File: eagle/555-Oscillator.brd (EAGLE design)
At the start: 27.9 x 30.5 mm, 8 parts, among them IC1 555

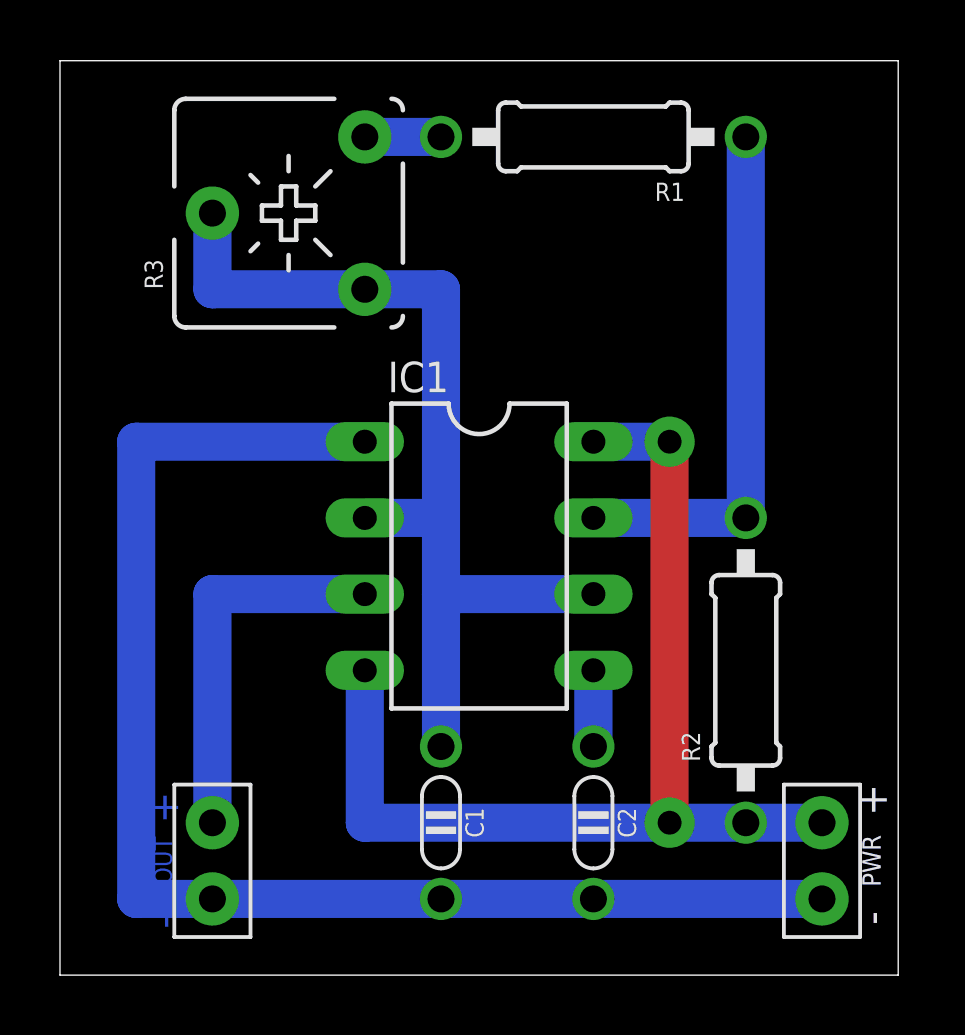
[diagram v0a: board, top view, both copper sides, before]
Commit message: ...
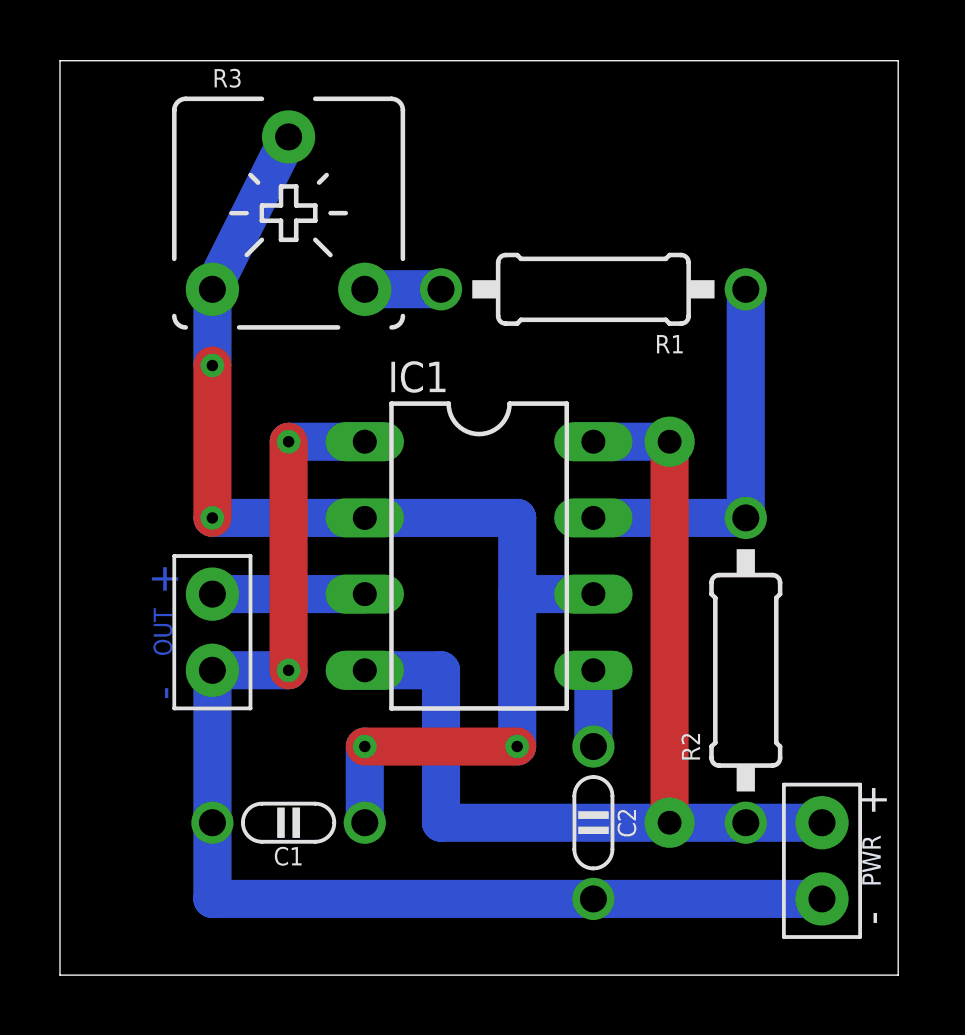
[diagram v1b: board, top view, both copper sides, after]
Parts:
- moved OUT 7.62 mm to (5.08, 11.4)
- moved R1 5.08 mm to (17.8, 22.9)
- moved C1 5.08 mm to (7.62, 5.08), turned to 90 degrees
- turned R3 to 0 degrees
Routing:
- net N$3: track 33.0 -> 41.2 mm, vias 0 -> 4
- net N$8: track 12.7 -> 5.08 mm
- net GND: track 45.7 -> 40.6 mm, vias 0 -> 2
- net N$1: track 17.8 -> 12.7 mm
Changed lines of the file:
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@@
 <layer number="24" name="bOrigins" color="15" fill="1" visible="yes" active="yes"/>
 <layer number="25" name="tNames" color="7" fill="1" visible="yes" active="yes"/>
-<layer number="26" name="bNames" color="7" fill="1" visible="no" active="yes"/>
+<layer number="26" name="bNames" color="7" fill="1" visible="yes" active="yes"/>
 <layer number="27" name="tValues" color="7" fill="1" visible="yes" active="yes"/>
-<layer number="28" name="bValues" color="7" fill="1" visible="no" active="yes"/>
+<layer number="28" name="bValues" color="7" fill="1" visible="yes" active="yes"/>
 <layer number="29" name="tStop" color="7" fill="3" visible="no" active="yes"/>
 <layer number="30" name="bStop" color="7" fill="6" visible="no" active="yes"/>
@@
 <layer number="46" name="Milling" color="3" fill="1" visible="no" active="yes"/>
 <layer number="47" name="Measures" color="7" fill="1" visible="no" active="yes"/>
-<layer number="48" name="Document" color="7" fill="1" visible="yes" active="yes"/>
+<layer number="48" name="Document" color="7" fill="1" visible="no" active="yes"/>
 <layer number="49" name="Reference" color="7" fill="1" visible="no" active="yes"/>
 <layer number="50" name="dxf" color="7" fill="1" visible="no" active="yes"/>
@@
 </autorouter>
 <elements>
-<element name="C1" library="c" package="C050-020X036/V" value="470n" x="12.7" y="5.08" rot="R180"/>
+<element name="C1" library="c" package="C050-020X036/V" value="470n" x="7.62" y="5.08" rot="R90"/>
 <element name="C2" library="c" package="C050-020X036/V" value="10n" x="17.78" y="5.08" rot="R180"/>
-<element name="OUT" library="pad" package="SPAD-+" value="SPAD+--+" x="5.08" y="3.81" rot="R180"/>
-<element name="R1" library="r" package="0207/10" value="1k" x="17.78" y="27.94" rot="R180"/>
+<element name="OUT" library="pad" package="SPAD-+" value="SPAD+--+" x="5.08" y="11.43" rot="R180"/>
+<element name="R1" library="r" package="0207/10" value="1k" x="17.78" y="22.86" rot="R180"/>
 <element name="R2" library="r" package="0207/10" value="10k" x="22.86" y="10.16" rot="R90"/>
-<element name="R3" library="r" package="POT-V" value="220k" x="7.62" y="25.4" rot="R90"/>
+<element name="R3" library="r" package="POT-V" value="220k" x="7.62" y="25.4"/>
 <element name="S1" library="pad" package="PWR-R" value="VCC_GNDPWR-R" x="25.4" y="3.81"/>
 <element name="IC1" library="ic" package="DIL08" value="555" x="13.97" y="13.97"/>
@@
 <contactref element="IC1" pad="7"/>
 <wire x1="17.78" y1="15.24" x2="22.86" y2="15.24" width="1.27" layer="16"/>
-<wire x1="22.86" y1="27.94" x2="22.86" y2="15.24" width="1.27" layer="16"/>
+<wire x1="22.86" y1="22.86" x2="22.86" y2="15.24" width="1.27" layer="16"/>
 </signal>
 <signal name="N$2">
 <contactref element="R1" pad="2"/>
 <contactref element="R3" pad="E"/>
-<wire x1="12.7" y1="27.94" x2="10.16" y2="27.94" width="1.27" layer="16"/>
+<wire x1="12.7" y1="22.86" x2="10.16" y2="22.86" width="1.27" layer="16"/>
 </signal>
 <signal name="N$3">
@@
 <contactref element="IC1" pad="6"/>
 <contactref element="IC1" pad="2"/>
-<wire x1="10.16" y1="22.86" x2="12.7" y2="22.86" width="1.27" layer="16"/>
-<wire x1="12.7" y1="22.86" x2="12.7" y2="15.24" width="1.27" layer="16"/>
-<wire x1="10.16" y1="15.24" x2="12.7" y2="15.24" width="1.27" layer="16"/>
-<wire x1="12.7" y1="15.24" x2="12.7" y2="12.7" width="1.27" layer="16"/>
-<wire x1="12.7" y1="12.7" x2="17.78" y2="12.7" width="1.27" layer="16"/>
-<wire x1="10.16" y1="22.86" x2="5.08" y2="22.86" width="1.27" layer="16"/>
-<wire x1="5.08" y1="22.86" x2="5.08" y2="25.4" width="1.27" layer="16"/>
-<wire x1="12.7" y1="7.62" x2="12.7" y2="12.7" width="1.27" layer="16"/>
+<wire x1="10.16" y1="15.24" x2="15.24" y2="15.24" width="1.27" layer="16"/>
+<wire x1="15.24" y1="15.24" x2="15.24" y2="12.7" width="1.27" layer="16"/>
+<wire x1="15.24" y1="12.7" x2="17.78" y2="12.7" width="1.27" layer="16"/>
+<wire x1="5.08" y1="22.86" x2="7.62" y2="27.94" width="1.27" layer="16"/>
+<wire x1="10.16" y1="15.24" x2="5.08" y2="15.24" width="1.27" layer="16"/>
+<via x="5.08" y="15.24" extent="1-16" drill="0.381"/>
+<wire x1="5.08" y1="15.24" x2="5.08" y2="20.32" width="1.27" layer="1"/>
+<via x="5.08" y="20.32" extent="1-16" drill="0.381"/>
+<wire x1="5.08" y1="20.32" x2="5.08" y2="22.86" width="1.27" layer="16"/>
+<wire x1="10.16" y1="5.08" x2="10.16" y2="7.62" width="1.27" layer="16"/>
+<via x="10.16" y="7.62" extent="1-16" drill="0.381"/>
+<wire x1="10.16" y1="7.62" x2="15.24" y2="7.62" width="1.27" layer="1"/>
+<via x="15.24" y="7.62" extent="1-16" drill="0.381"/>
+<wire x1="15.24" y1="7.62" x2="15.24" y2="12.7" width="1.27" layer="16"/>
 </signal>
 <signal name="GND">
@@
 <contactref element="C2" pad="2"/>
 <contactref element="OUT" pad="1"/>
-<wire x1="10.16" y1="17.78" x2="2.54" y2="17.78" width="1.27" layer="16"/>
-<wire x1="2.54" y1="17.78" x2="2.54" y2="2.54" width="1.27" layer="16"/>
-<wire x1="2.54" y1="2.54" x2="5.08" y2="2.54" width="1.27" layer="16"/>
-<wire x1="5.08" y1="2.54" x2="12.7" y2="2.54" width="1.27" layer="16"/>
-<wire x1="12.7" y1="2.54" x2="17.78" y2="2.54" width="1.27" layer="16"/>
+<wire x1="10.16" y1="17.78" x2="7.62" y2="17.78" width="1.27" layer="16"/>
+<wire x1="7.62" y1="17.78" x2="7.62" y2="10.16" width="1.27" layer="1"/>
+<wire x1="7.62" y1="10.16" x2="5.08" y2="10.16" width="1.27" layer="16"/>
+<wire x1="5.08" y1="10.16" x2="5.08" y2="5.08" width="1.27" layer="16"/>
+<wire x1="5.08" y1="5.08" x2="5.08" y2="2.54" width="1.27" layer="16"/>
+<wire x1="5.08" y1="2.54" x2="17.78" y2="2.54" width="1.27" layer="16"/>
 <wire x1="25.4" y1="2.54" x2="17.78" y2="2.54" width="1.27" layer="16"/>
+<via x="7.62" y="17.78" extent="1-16" drill="0.381"/>
+<via x="7.62" y="10.16" extent="1-16" drill="0.381"/>
 </signal>
 <signal name="N$6">
@@
 <contactref element="IC1" pad="4"/>
 <contactref element="R2" pad="1"/>
-<wire x1="10.16" y1="10.16" x2="10.16" y2="5.08" width="1.27" layer="16"/>
-<wire x1="10.16" y1="5.08" x2="20.32" y2="5.08" width="1.27" layer="16"/>
+<wire x1="10.16" y1="10.16" x2="12.7" y2="10.16" width="1.27" layer="16"/>
+<wire x1="12.7" y1="10.16" x2="12.7" y2="5.08" width="1.27" layer="16"/>
+<wire x1="12.7" y1="5.08" x2="20.32" y2="5.08" width="1.27" layer="16"/>
 <wire x1="20.32" y1="5.08" x2="22.86" y2="5.08" width="1.27" layer="16"/>
 <wire x1="25.4" y1="5.08" x2="22.86" y2="5.08" width="1.27" layer="16"/>
@@
 <contactref element="OUT" pad="2"/>
 <contactref element="IC1" pad="3"/>
-<wire x1="5.08" y1="5.08" x2="5.08" y2="12.7" width="1.27" layer="16"/>
 <wire x1="5.08" y1="12.7" x2="10.16" y2="12.7" width="1.27" layer="16"/>
 </signal>
